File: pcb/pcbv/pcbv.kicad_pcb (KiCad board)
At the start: 4 copper layers, 55 x 72 mm, 41 parts, among them J1 Conn_ST_STDC14, J2 I2C, J4 CAN+POWER, J5 CAN, J6 3.3V, J7 5V, SW1 generic 6mm tht switch, U1 MPRLS0025PA00001A, U2 STM32C092RCT6, U3 SCD40-D-R2, U4 LV2862YDDC, U5 TLV709A50DBZR, U6 TJA1051T-3, Y1 48MHz, Y2 32.768KHz

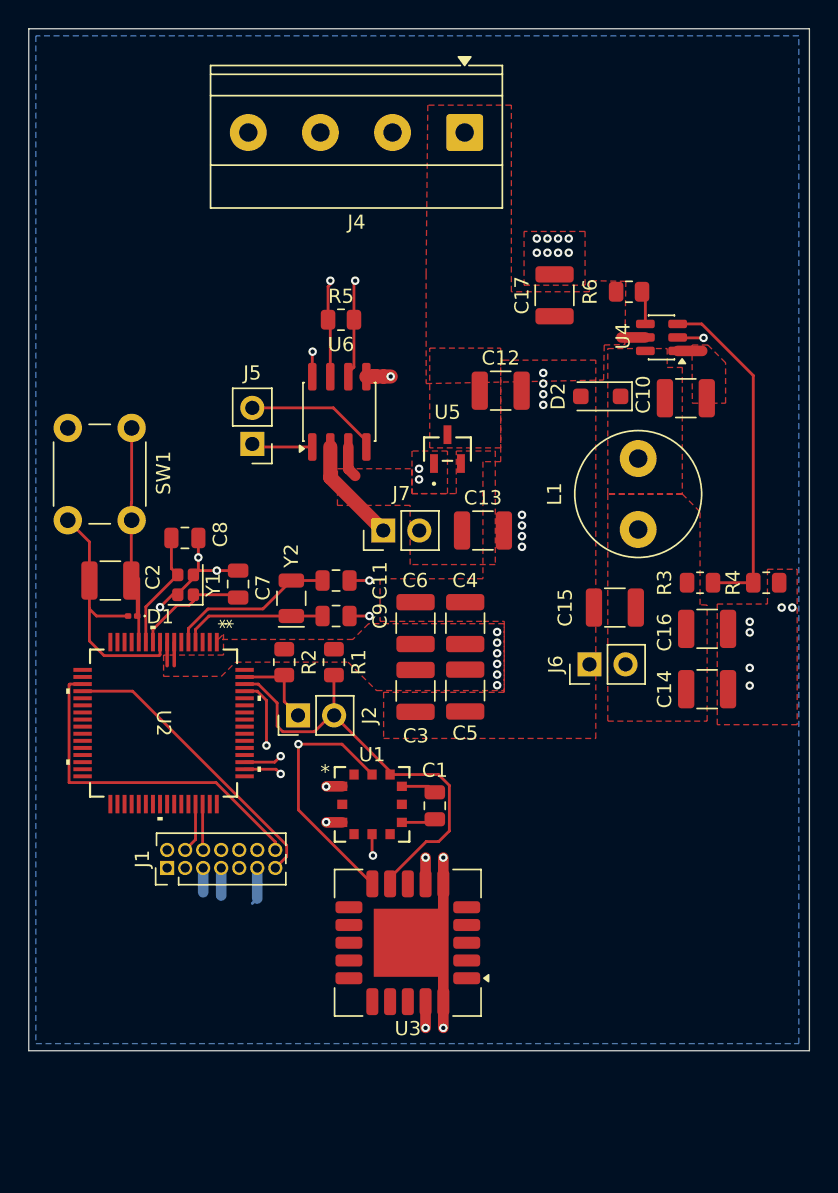
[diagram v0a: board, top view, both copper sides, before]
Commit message: pcb updated
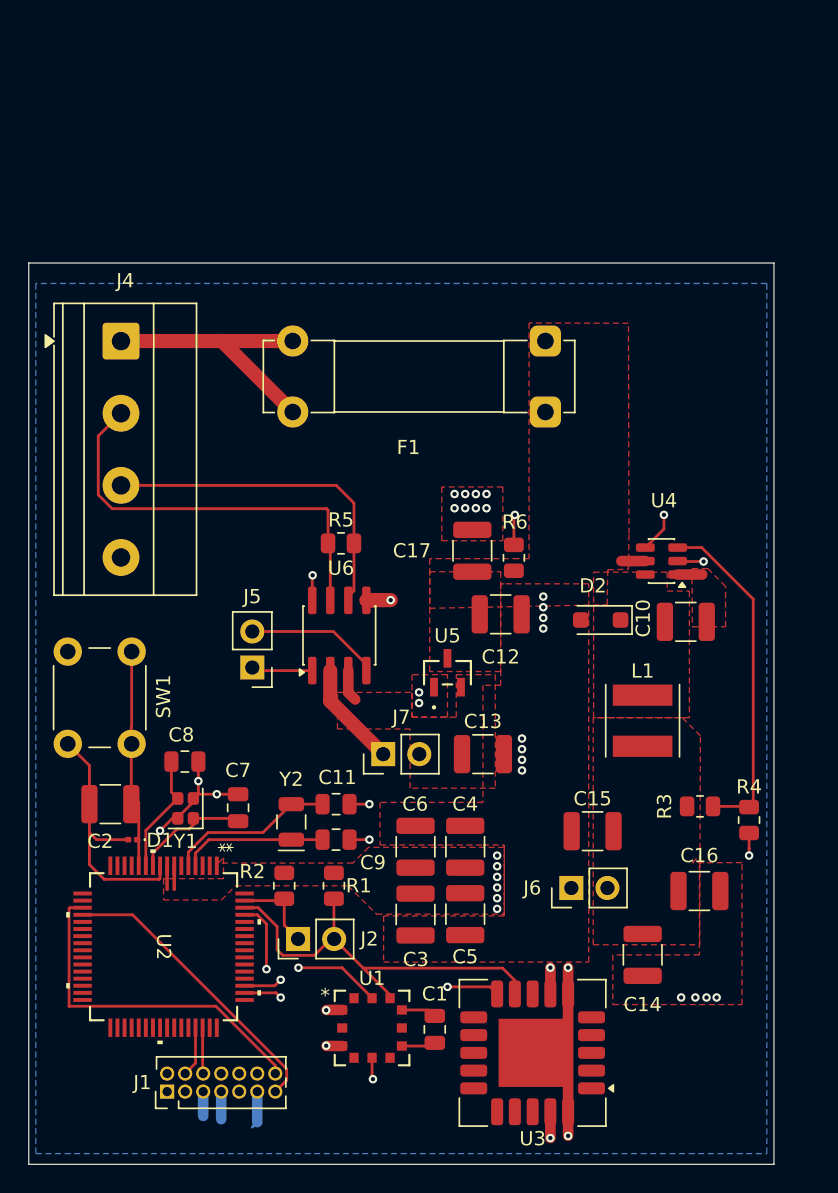
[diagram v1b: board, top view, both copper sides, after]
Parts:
- added F1: Fuse, Fuse:Fuseholder_Clip-5x20mm_Bel_FC-203-22_Lateral_P17.80x5.00mm_D1.17mm_Horizontal, F.Cu at (98.7, 39.8)
- D1: value ESDZL5 -> ESDZL5-1F4
- L1: value 18u-RLB0914-180KL -> 18u; footprint Inductor_THT:L_Radial_D8.7mm_P5.00mm_Fastron_07HCP -> Inductor_SMD:L_Taiyo-Yuden_MD-5050
- U4: value LV2862YDDC -> LV2862YDDCT
- U5: value TLV709A50DBZR -> TLV709A50DBVR
- moved J4 28.3 mm to (68.8, 34.8), turned to -90 degrees
- moved R6 20.4 mm to (96.4, 50.0), turned to -90 degrees
- moved C14 19.3 mm to (105.5, 78.0), turned to -90 degrees
- moved C17 18.9 mm to (93.5, 49.5)
- moved C16 18.5 mm to (109.5, 73.5)
- moved L1 18.5 mm to (105.5, 61.5)
- moved R4 16.8 mm to (113.0, 68.5), turned to 90 degrees
- moved C15 15.8 mm to (102.0, 69.3)
- moved J6 15.8 mm to (100.5, 73.3)
- moved C1 15.8 mm to (90.9, 83.2)
- moved U1 15.8 mm to (86.4, 83.1)
- moved C3 15.8 mm to (89.5, 75.2)
- moved D2 15.8 mm to (102.5, 54.4)
- moved U2 15.8 mm to (71.8, 77.4)
- moved U5 15.8 mm to (91.8, 58.1)
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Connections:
- J4 pad 1: VDD -> Net-(J4-Pin_1)
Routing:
- net Net-(J4-Pin_1): track 0.00 -> 19.2 mm
- net Net-(U4-~{SHDN}): track 2.36 -> 16.1 mm, vias 0 -> 2
- net /CANH: track 21.2 -> 29.5 mm, vias 1 -> 0
- net /CANL: track 18.6 -> 24.2 mm, vias 1 -> 0
- net /SDA: track 26.2 -> 29.0 mm, vias 1 -> 2
- net /NRST: track 45.0 -> 42.9 mm
- net /SCL: track 31.5 -> 29.8 mm
- net GND: track 61.7 -> 62.7 mm, vias 34 -> 33
- removed copper zone on In1.Cu, net GND
- removed copper zone on In2.Cu, net GND
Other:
- board size 55 x 72 mm -> 52.5 x 63.5 mm
